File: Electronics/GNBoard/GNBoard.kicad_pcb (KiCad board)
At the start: 2 copper layers, 77.9 x 54.5 mm, 47 parts, among them K1 IR1, K10 IR4, K11 CNY_1, K12 CNY_2, K13 CNY_3, K14 CNY_4, K15 CNY_5, K16 CNY_6, K2 IR2, K3 SERVO_1, K4 SERVO_2, K5 SERVO_3, K6 SERVO_4, K7 SERVO_5, K8 SERVO_6, K9 IR3, P1 Battery, P2 CONN_5, P3 Spk, P4 I2C_1, P5 I2C_2, P6 DHT_Conn, SW1 PowerSwitch, SW2 SW_PUSH, SW3 SW_PUSH, U1 LM2576

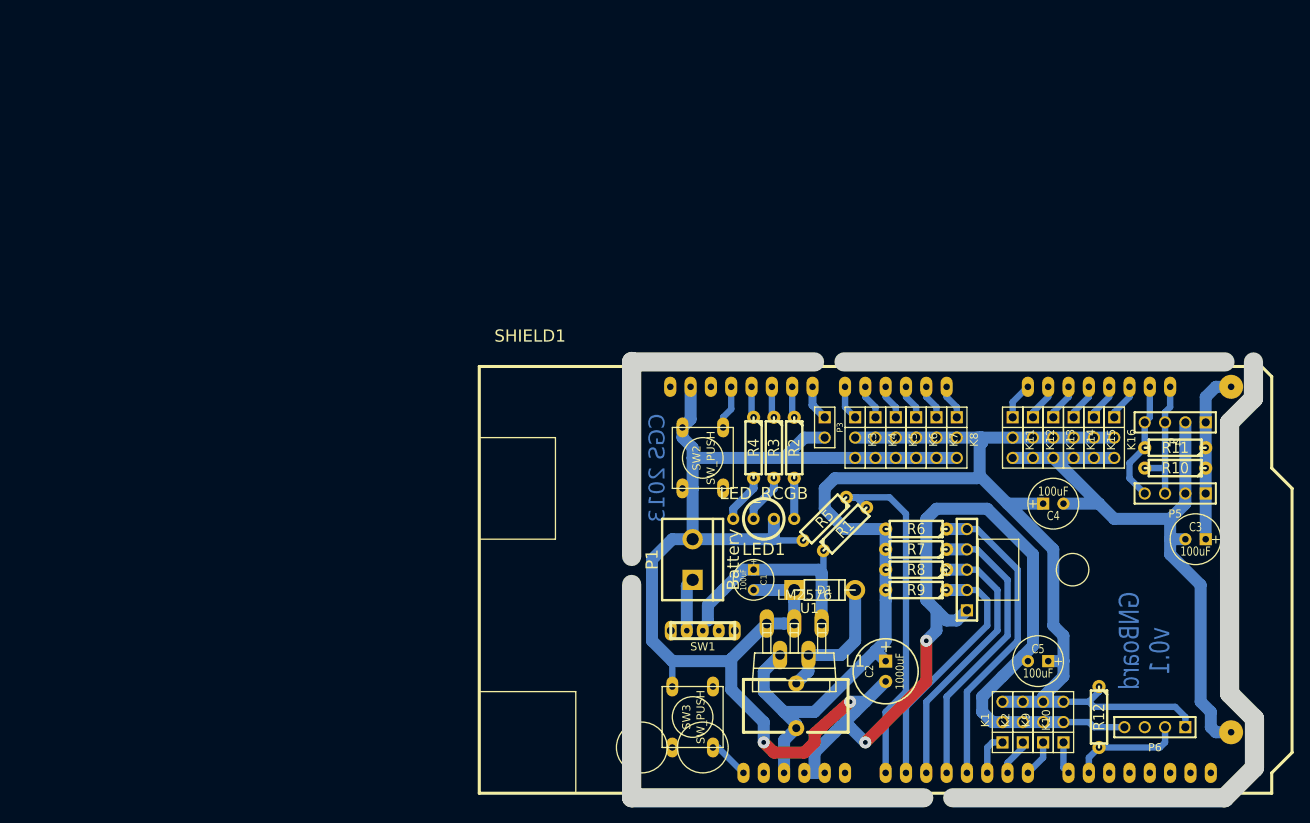
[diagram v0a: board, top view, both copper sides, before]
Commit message: Working in new version for the GNBoard
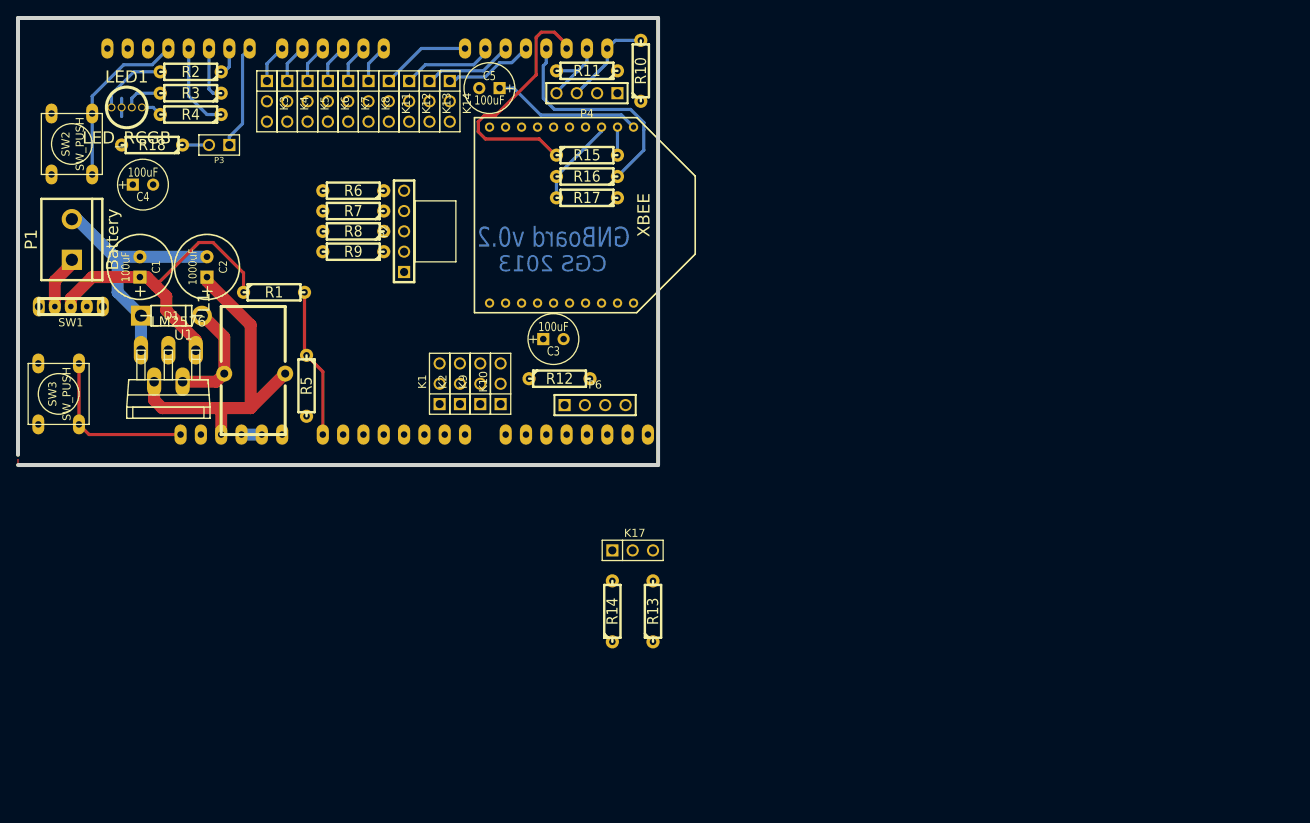
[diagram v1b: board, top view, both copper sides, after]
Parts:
- removed K15: CNY_5, PIN_ARRAY_3X1
- removed K16: CNY_6, PIN_ARRAY_3X1
- removed P5: I2C_2, PIN_ARRAY_4x1
- added K17: Nose, PIN_ARRAY_3X1, F.Cu at (125.9, 92.8)
- added M1: XBEE, xbee_r1-XBEE, F.Cu at (117.0, 50.9)
- added R13: 10k, R3-LARGE_PADS, F.Cu at (128.4, 100.5)
- added R14: 10k, R3-LARGE_PADS, F.Cu at (123.3, 100.5)
- added R15: 4k7, R3-LARGE_PADS, F.Cu at (120.1, 43.4)
- added R16: 4k7, R3-LARGE_PADS, F.Cu at (120.1, 46.1)
- added R17: 7k5, R3-LARGE_PADS, F.Cu at (120.1, 48.8)
- added R18: 99k, R3-LARGE_PADS, F.Cu at (65.8, 42.2)
- C1: footprint C1V5 -> C1V8
- L1: footprint Choke_Toroid_6,5x13mm_Vertical -> Choke_Toroid_8x16mm_Vertical
- LED1: footprint LED5_RGB_long_wide -> LED5_RGB_long
- R1: value 6k8 -> 62k
- R5: value 6k8 -> 20k
- SHIELD1: footprint ARDUINO_MEGA_SHIELD -> ARDUINO_MEGA_SHIELD_MOD
- SW1: footprint SWITCH_3Pin -> switch_power_custom
- moved C4 120.6 mm to (64.6, 47.1)
- moved C5 99.2 mm to (108.0, 35.1)
- moved C2 98.8 mm to (72.6, 57.4), turned to 90 degrees
- moved LED1 94.8 mm to (62.6, 37.5), turned to 0 degrees
- moved SW3 88.9 mm to (54.1, 73.3)
- moved R2 88.9 mm to (70.6, 33.0), turned to 180 degrees
- moved SW1 88.8 mm to (55.6, 62.4)
- moved K11 88.6 mm to (95.4, 36.7)
- moved K12 88.6 mm to (97.9, 36.7)
- moved K13 88.6 mm to (100.5, 36.7)
- moved K14 88.6 mm to (103.0, 36.7)
- moved D1 88.6 mm to (68.2, 63.5)
- moved SW2 88.1 mm to (55.8, 42.0)
- moved R11 87.3 mm to (120.1, 32.9)
- moved P1 87.3 mm to (55.8, 54.0)
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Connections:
- C5 pad 1: +5V -> +3.3V
- P3 pad 2: GND -> N-0000043
- P6 pad 3: N-0000082 -> (no net)
- SHIELD1 pad 13: N-0000067 -> (no net)
- SHIELD1 pad 18: CNY5 -> XB_DIN
- SHIELD1 pad 19: CNY6 -> XB_DOUT
- SHIELD1 pad 3V3: N-0000040 -> +3.3V
- SHIELD1 pad AD10: N-0000041 -> Nose_V
- SHIELD1 pad AD11: N-0000039 -> (no net)
- SHIELD1 pad AD12: N-0000042 -> (no net)
- SHIELD1 pad AD13: N-0000043 -> (no net)
- SHIELD1 pad AD14: N-0000044 -> (no net)
- SHIELD1 pad AD15: N-0000045 -> (no net)
- SHIELD1 pad AREF: N-0000037 -> (no net)
- SHIELD1 pad V_IN: N-0000038 -> (no net)
- SW1 pad 3: N-0000046 -> (no net)
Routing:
- net GND: track 352.1 -> 36.9 mm, vias 4 -> 0
- net +5V: track 208.7 -> 43.3 mm
- net LDR4: track 39.0 -> 0.00 mm
- net LDR3: track 36.5 -> 0.00 mm
- net LDR2: track 33.9 -> 0.00 mm
- net XB_DOUT: track 0.00 -> 31.8 mm
- net LDR1: track 31.4 -> 0.00 mm
- net XB_DIN: track 0.00 -> 28.3 mm
- net BattVolt: track 44.8 -> 18.7 mm
- net +3.3V: track 0.00 -> 18.8 mm
- net Button1: track 5.50 -> 21.8 mm
- net ResetB: track 5.13 -> 20.8 mm
- net DHTpin: track 14.1 -> 0.00 mm
- net +BATT: track 28.9 -> 40.5 mm
- net N-0000034: track 0.00 -> 11.2 mm
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- added copper zone on F.Cu, net +5V
- added copper zone on B.Cu, net GND
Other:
- board size 77.9 x 54.5 mm -> 80 x 55.9 mm
- net class Default: clearance 0.4 -> 0.3; trace_width 0.8 -> 0.4; via_dia 1.5 -> 0.889; via_drill 0.6 -> 0.508
- rule trace_clearance: 0.4 -> 0.3
- board text added: "GNBoard v0.2"
- board text removed: "GNBoard"
- board text removed: "v0.1"
